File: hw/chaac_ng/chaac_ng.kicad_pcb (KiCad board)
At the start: 4 copper layers, 32 x 66 mm, 76 parts, among them J1 Battery, J2 Solar, J3 TC2030-CTX, J4 Conn_01x04, J5 USB_C_Receptacle_USB2.0_16P, SW1 SW_Push, SW2 SW_Push, U1 E22-X00M22S, U2 BQ24074RGT, U3 TPS76333, U4 MAX3221, U5 STM32L412KBTx, U6 TPS61252DSG, Y1 32.768kHz

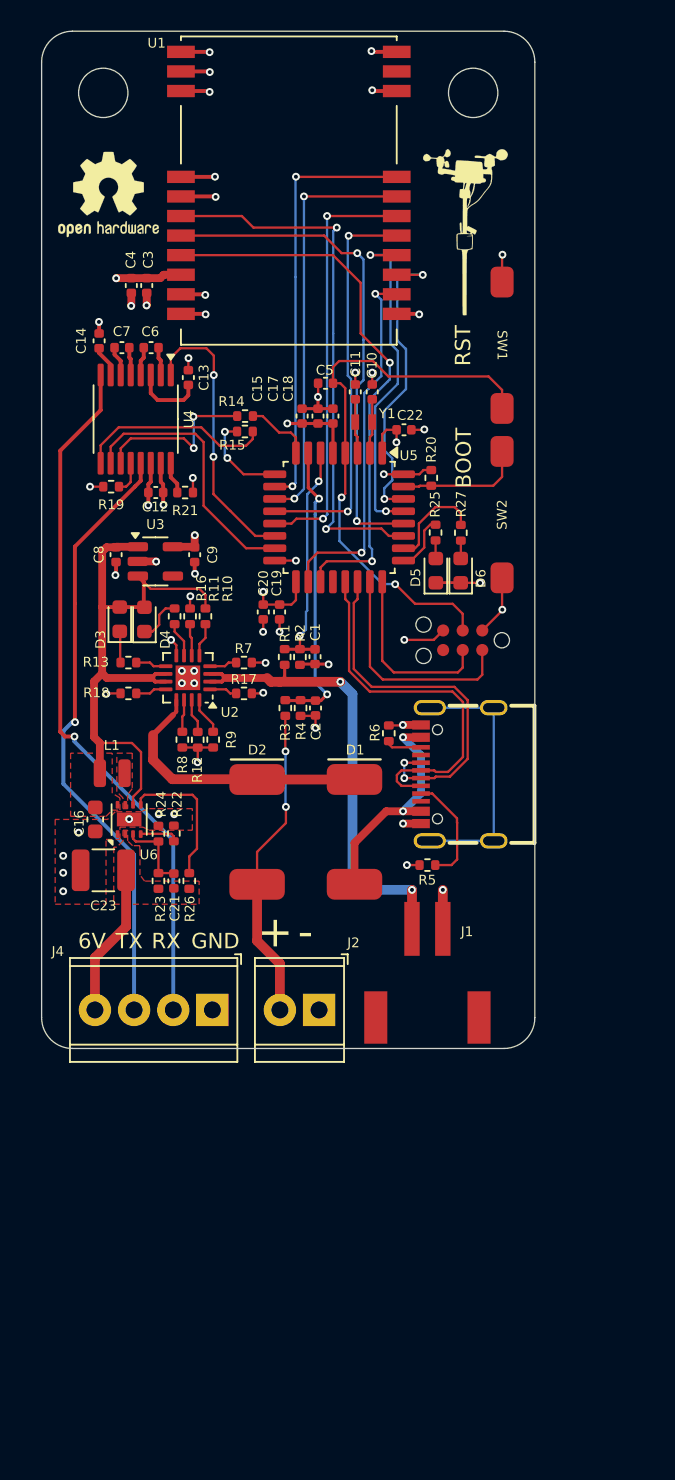
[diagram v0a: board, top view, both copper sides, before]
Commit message: Chaac ng 7.1
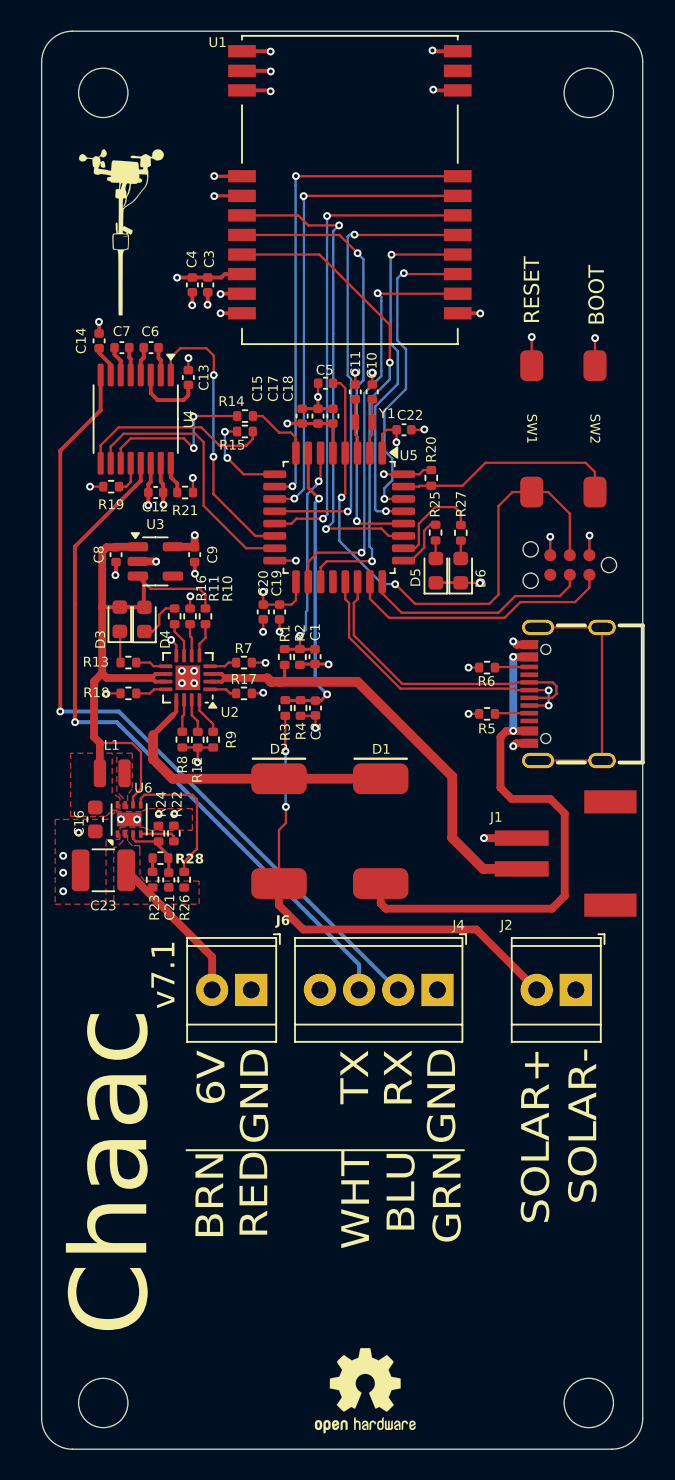
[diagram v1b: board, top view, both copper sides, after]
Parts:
- added H3: MountingHole, MountingHole:MountingHole_3.2mm_M3, F.Cu at (116.5, 159.0)
- added H4: MountingHole, MountingHole:MountingHole_3.2mm_M3, F.Cu at (85.0, 159.0)
- added H5: MountingHole, alvarop:ZIPTIE_HOLE_4x2mm, F.Cu at (92.8, 151.0)
- added H6: MountingHole, alvarop:ZIPTIE_HOLE_4x2mm, F.Cu at (105.2, 151.0)
- added H7: MountingHole, alvarop:ZIPTIE_HOLE_4x2mm, F.Cu at (110.2, 151.0)
- added H8: MountingHole, alvarop:ZIPTIE_HOLE_4x2mm, F.Cu at (117.6, 151.0)
- added J6: 6V_PWR, alvarop:TerminalBlock_TE_282834-2_1x02_P2.54mm_Horizontal, F.Cu at (94.6, 132.2)
- added R28: 43k, Resistor_SMD:R_0402_1005Metric, F.Cu at (88.7, 123.7)
- J4: value Conn_01x04 -> DATA
- R23: value 715k -> 750k
- moved REF** 79.4 mm to (102.0, 158.2)
- moved G*** 22.3 mm to (86.2, 83.0)
- moved J2 16.7 mm to (115.7, 132.2)
- moved J4 14.7 mm to (106.7, 132.2)
- moved R5 10.5 mm to (109.9, 114.3)
- moved J5 8.75 mm to (115.0, 113.0)
- moved J3 8.49 mm to (115.3, 104.6)
- moved SW2 8.20 mm to (116.9, 95.8), turned to -90 degrees
- moved J1 7.83 mm to (112.2, 123.3), turned to -90 degrees
- moved R6 7.67 mm to (109.9, 111.3), turned to 180 degrees
- moved H2 7.50 mm to (116.5, 74.0)
- moved SW1 5.76 mm to (112.8, 95.8)
- moved G*** 4.07 mm to (101.4, 109.6)
- moved C3 3.96 mm to (91.8, 86.5)
- moved C4 3.96 mm to (90.8, 86.5)
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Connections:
- J4 pad 4: +6V -> unconnected-(J4-Pin_4-Pad4)
- R19 pad 2: +3.3V -> GND
- R21 pad 1: GND -> +3.3V
- R23 pad 2: Net-(U6-FB) -> Net-(R23-Pad2)
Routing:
- net VBUS: track 14.8 -> 35.1 mm
- net /SOLAR_IN: track 20.5 -> 31.5 mm
- net /RS232_RX: track 45.7 -> 52.3 mm
- net /BOOT: track 8.31 -> 14.6 mm
- net /RS232_TX: track 39.6 -> 45.2 mm
- net Net-(J5-CC1): track 7.24 -> 2.25 mm
- net /RADIO_DIO2: track 36.4 -> 32.0 mm
- net /USB_DN: track 24.6 -> 20.3 mm, vias 0 -> 2
- net /SCK: track 27.2 -> 31.2 mm
- net /RADIO_CS: track 27.9 -> 31.9 mm
- net /MISO: track 26.0 -> 30.0 mm
- net /USB_DP: track 24.5 -> 20.5 mm, vias 2 -> 0
- net /MOSI: track 27.5 -> 31.5 mm
- net /RADIO_TXEN: track 32.7 -> 28.8 mm
- net /RADIO_DIO1: track 23.9 -> 27.7 mm
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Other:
- board size 32 x 66 mm -> 39 x 92 mm
- board text added: "BLU"
- board text added: "BRN"
- board text added: "GRN"
- board text added: "RED"
- board text added: "RESET"
- board text added: "SOLAR+"
- board text added: "SOLAR-"
- board text added: "WHT"
- board text removed: "+"
- board text removed: "-"
- board text removed: "RST"
